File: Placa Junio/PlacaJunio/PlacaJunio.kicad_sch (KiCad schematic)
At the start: 12 parts, among them IC1 LC86LICMD, J1 Bateria, Q4 IRLML0030, U5 TSR2-2433N

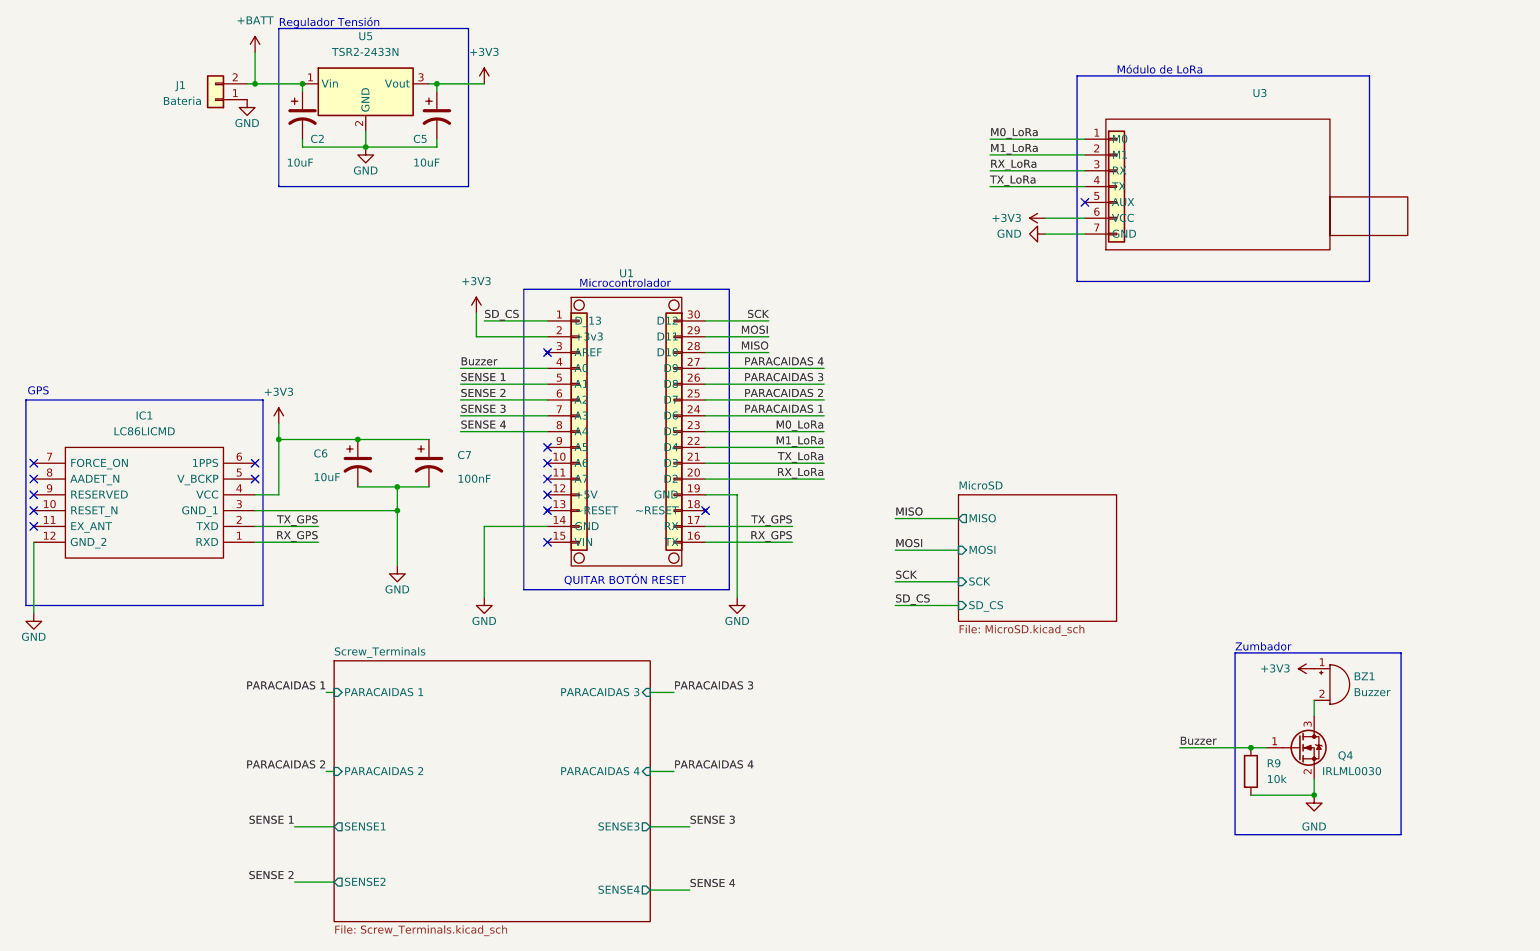
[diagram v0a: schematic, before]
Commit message: Esquemático Completo
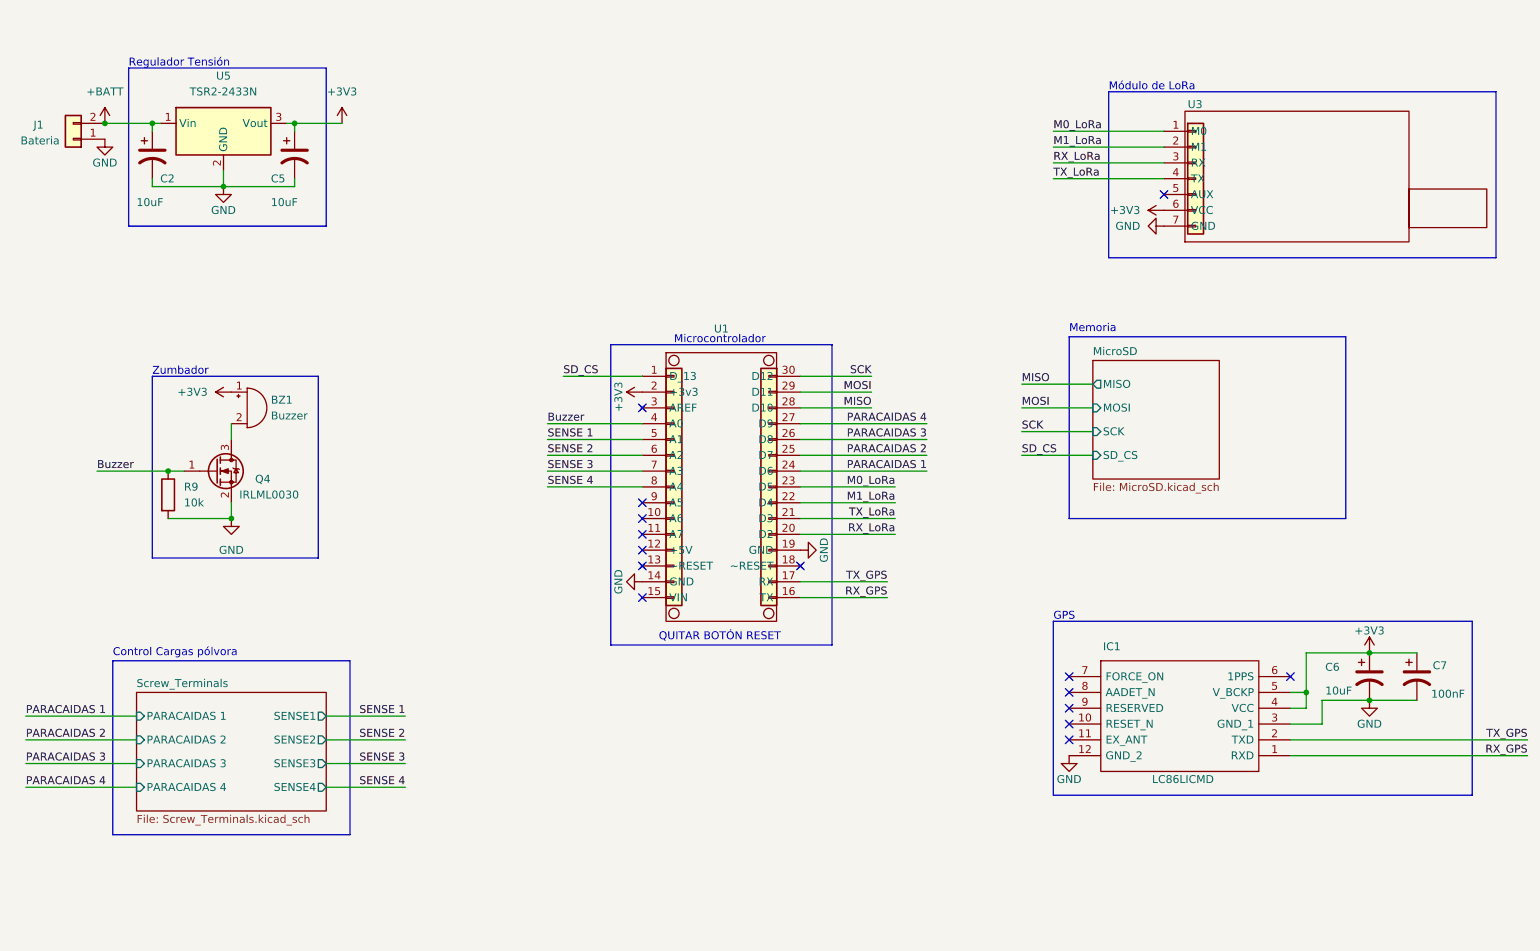
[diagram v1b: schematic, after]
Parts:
- U1: footprint (none) -> Cohete_Julio:Nano BLE 33 Sense
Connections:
- net +3V3: now also IC1.5 (V_BCKP)
- no-connect marks 16 -> 15
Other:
- note added: "Control Cargas pólvora"
- note added: "Memoria"
- moved on the sheet: BZ1, C2, C5, C6, C7, IC1, J1, Q4, R9, U3, U5
